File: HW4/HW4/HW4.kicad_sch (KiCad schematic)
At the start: 5 parts, among them J1 Conn_01x12_Pin, U1 AP7384-33V

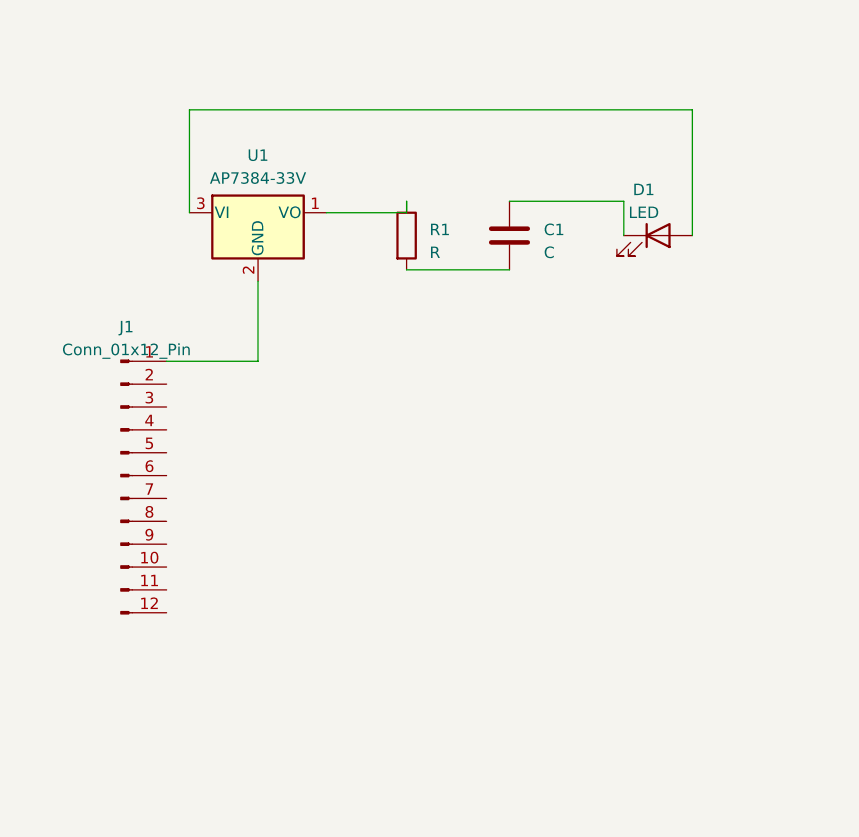
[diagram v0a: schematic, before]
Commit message: idk what happened lol
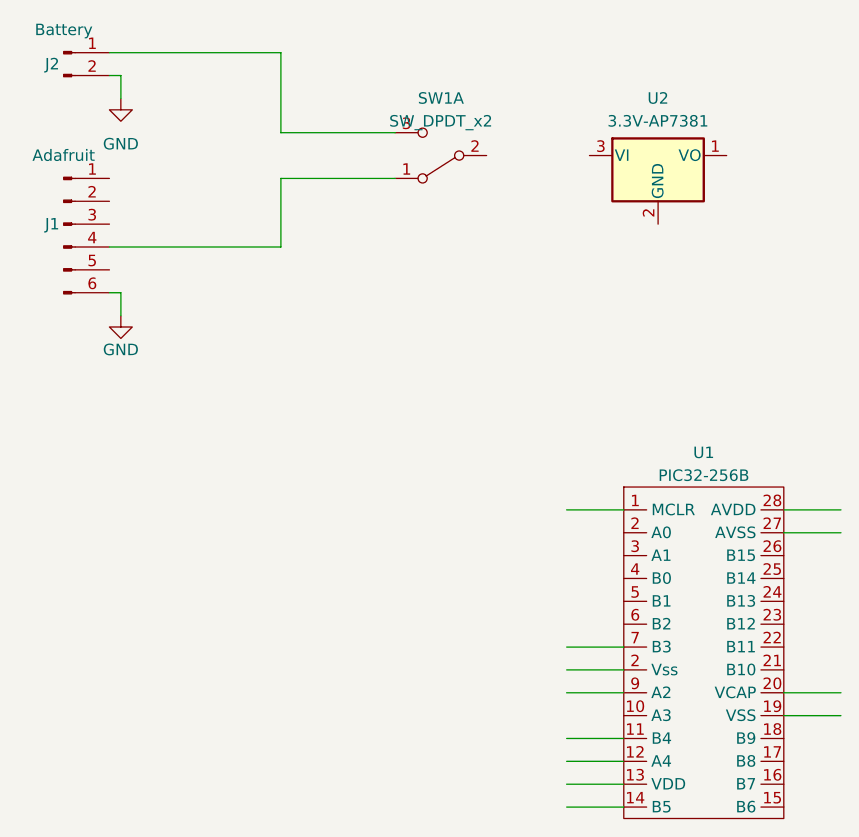
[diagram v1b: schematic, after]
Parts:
- removed C1: C, Capacitor_THT:C_Disc_D3.4mm_W2.1mm_P2.50mm, symbol Device:C
- removed D1: LED, LED_THT:LED_D3.0mm, symbol Device:LED
- removed J1: Conn_01x12_Pin, symbol Connector:Conn_01x12_Pin
- removed R1: R, Resistor_THT:R_Axial_DIN0207_L6.3mm_D2.5mm_P7.62mm_Horizontal, symbol Device:R
- removed U1: AP7384-33V, Package_TO_SOT_THT:TO-92L_Inline, symbol ME433-HW4:AP7384-33V
- added J1: Adafruit, symbol Connector:Conn_01x06_Pin
- added J2: Battery, symbol Connector:Conn_01x02_Pin
- added SW1: SW_DPDT_x2, symbol ME433-HW4:SW_DPDT_x2
- added U1: PIC32-256B, symbol ME433-HW4:PIC32-256B
- added U2: 3.3V-AP7381, symbol ME433-HW4:3.3V-AP7381
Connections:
- new net: J1.4 (Pin_4), SW1.1 (A)
- new net: J2.1 (Pin_1), SW1.3 (C)
- new net GND: J1.6 (Pin_6), J2.2 (Pin_2)
